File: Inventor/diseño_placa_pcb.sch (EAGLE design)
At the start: 14 parts, among them IC2 7805T

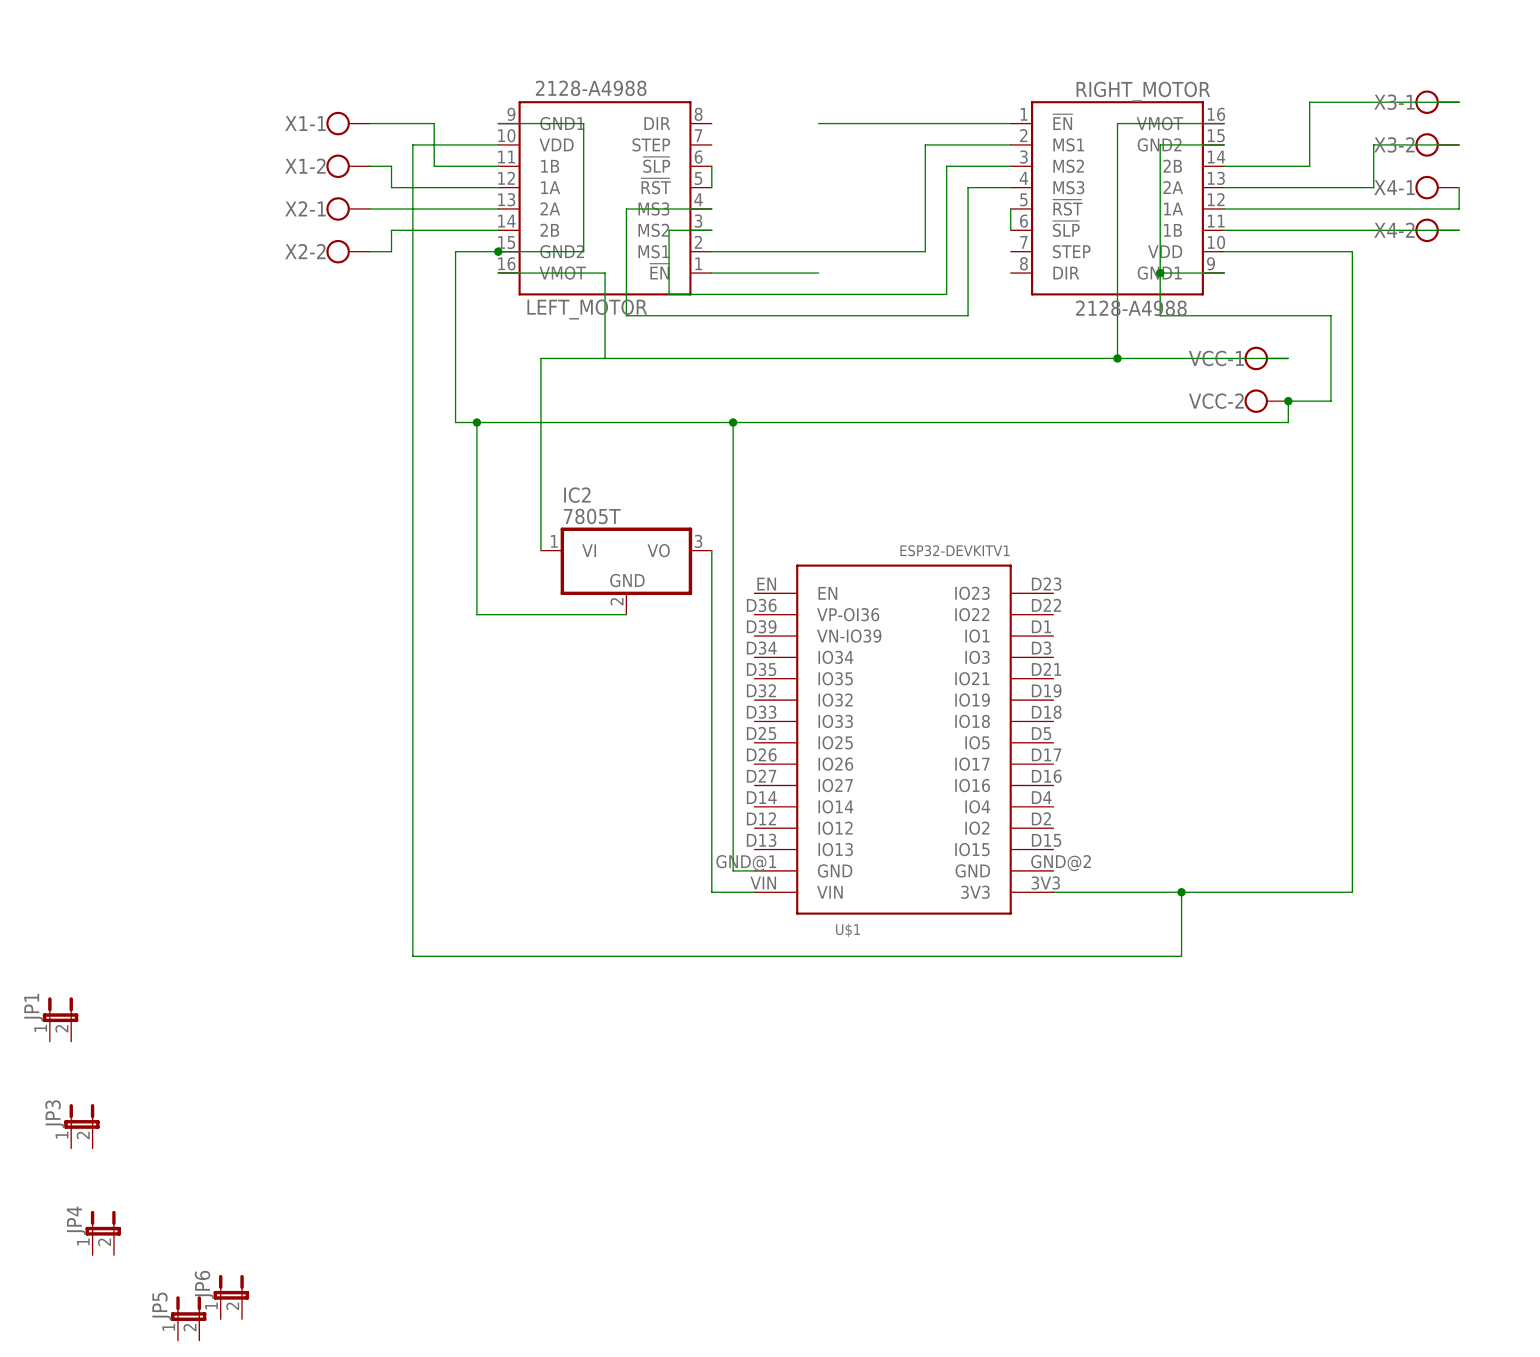
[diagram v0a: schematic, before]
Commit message: pcb_design
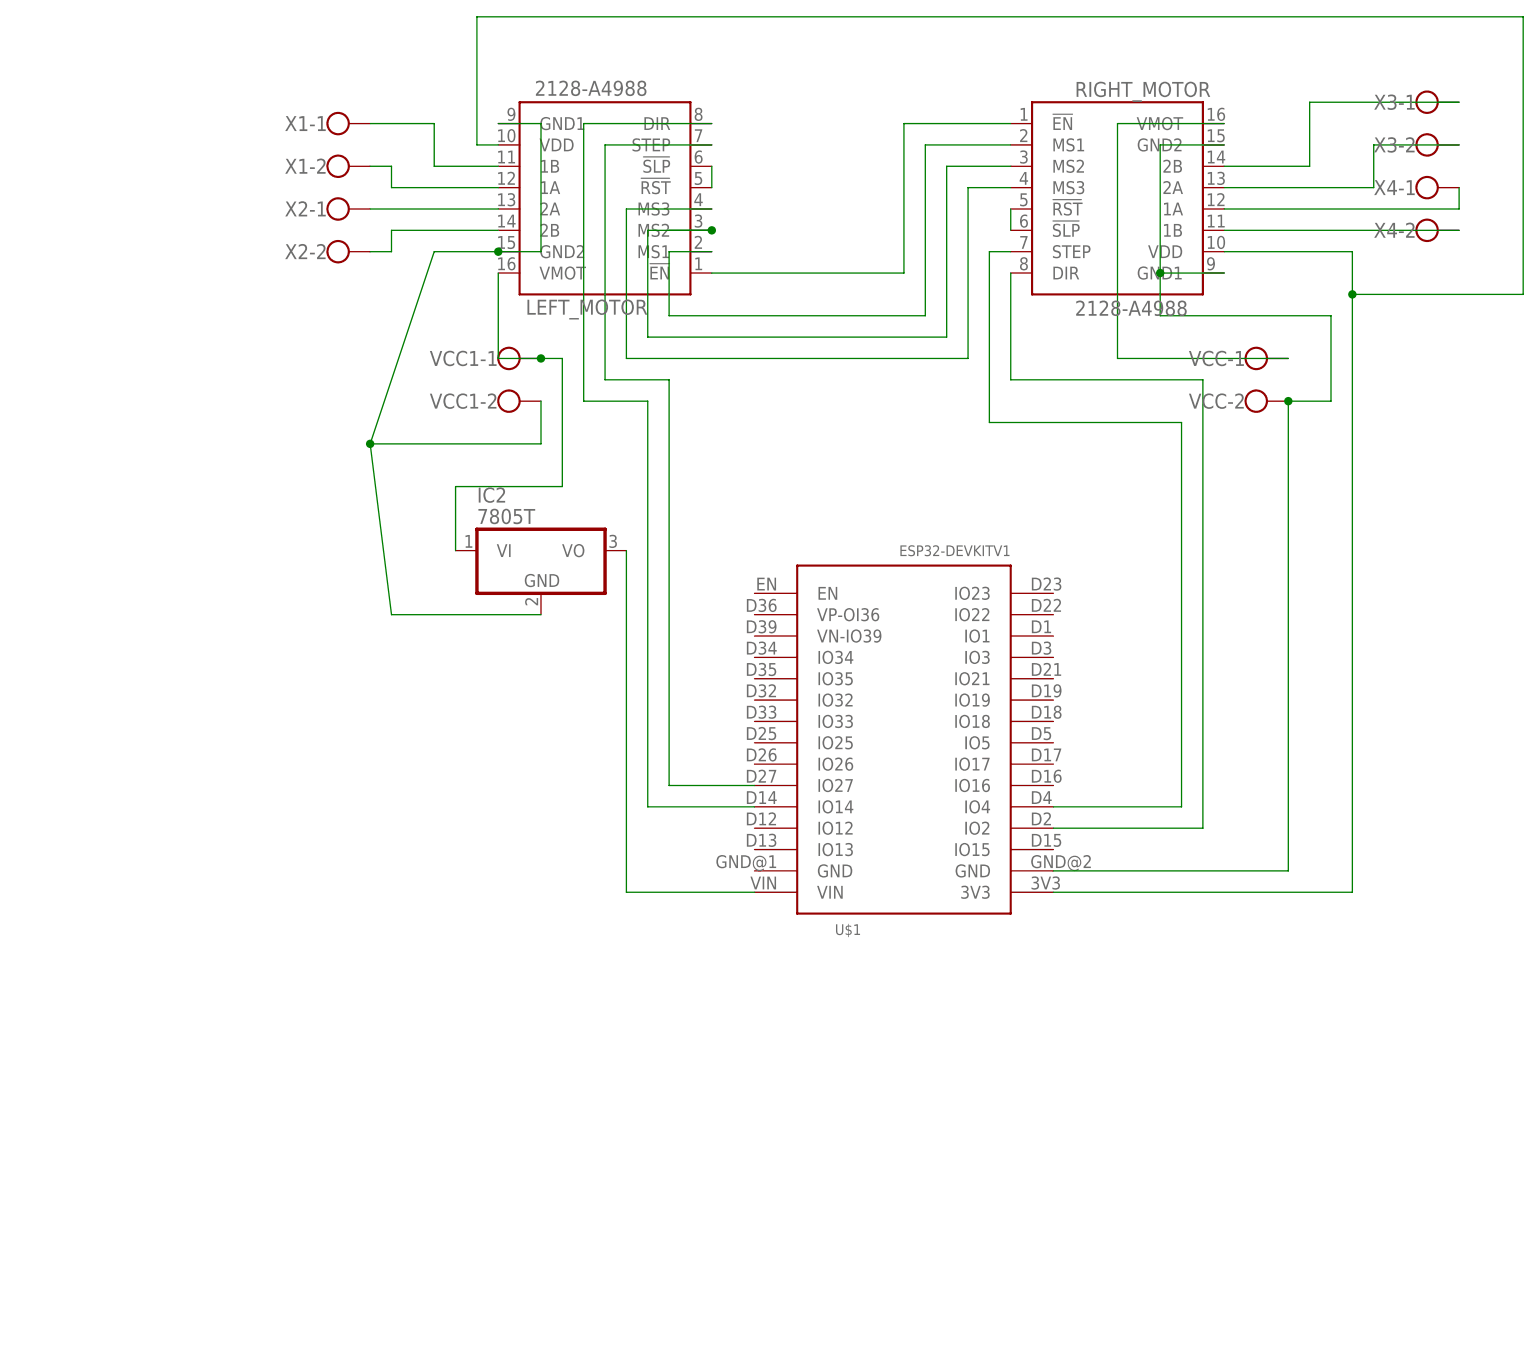
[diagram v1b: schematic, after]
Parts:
- removed JP1, JP3, JP4, JP5, JP6: (no value), jumper:JP1E
- added VCC1: (no value), con-wago-500:W237-102
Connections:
- new net N$20: LEFT_MOTOR.DIR, U$1.IO14
- new net N$21: IC2.VI, LEFT_MOTOR.VMOT, VCC1-1.KL
- new net N$22: RIGHT_MOTOR.GND1, RIGHT_MOTOR.GND2, U$1.GND@2, VCC-2.KL
- new net N$24: IC2.GND, LEFT_MOTOR.GND1, LEFT_MOTOR.GND2, VCC1-2.KL
- new net N$9: RIGHT_MOTOR.STEP, U$1.IO4
- net N$10: no longer IC2.VI, LEFT_MOTOR.VMOT
- net N$12: now also LEFT_MOTOR.!EN
- net N$14: now also LEFT_MOTOR.STEP, U$1.IO27; no longer LEFT_MOTOR.!EN
- net N$6: now also RIGHT_MOTOR.DIR, U$1.IO2; no longer IC2.GND, LEFT_MOTOR.GND1, LEFT_MOTOR.GND2, RIGHT_MOTOR.GND1, RIGHT_MOTOR.GND2, U$1.GND@1, VCC-2.KL
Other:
- moved on the sheet: IC2
